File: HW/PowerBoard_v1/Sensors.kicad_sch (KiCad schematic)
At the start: 46 parts, among them U3 MCP9700AT-ETT, U4 PAMC1350DWVR, U5 PAMC1350DWVR, U6 PAMC1350DWVR, U7 PAMC1350DWVR, U8 3v3 ISO DC/DC

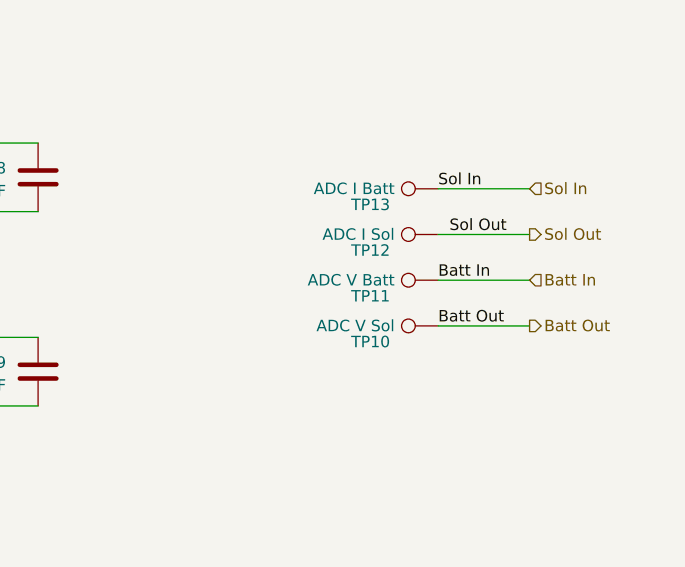
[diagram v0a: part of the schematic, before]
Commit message: pushed board
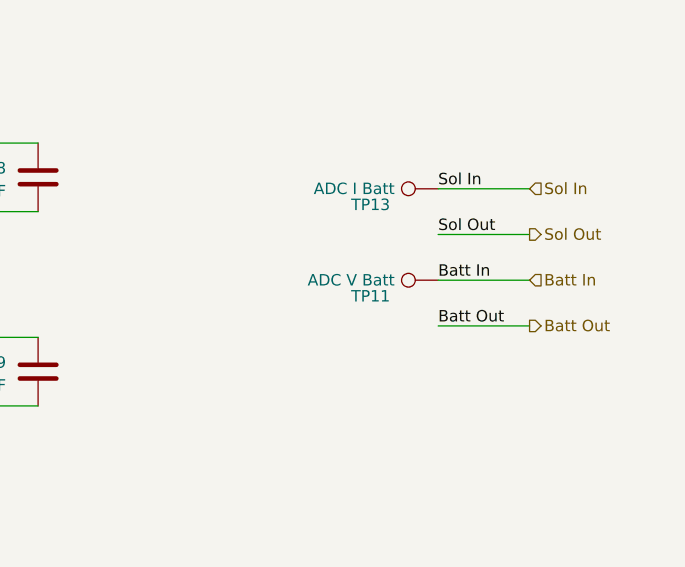
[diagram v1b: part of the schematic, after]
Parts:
- removed TP10: ADC V Sol, TestPoint:TestPoint_THTPad_1.0x1.0mm_Drill0.5mm, symbol Connector:TestPoint
- removed TP12: ADC I Sol, TestPoint:TestPoint_THTPad_1.0x1.0mm_Drill0.5mm, symbol Connector:TestPoint
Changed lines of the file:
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@@
 		)
 	)
-	(wire
-		(pts
-			(xy 245.11 129.54) (xy 255.27 129.54)
-		)
-		(stroke
-			(width 0)
-			(type default)
-		)
-	)
 	(polyline
 		(pts
@@
 	(wire
 		(pts
+			(xy 245.11 129.54) (xy 255.27 129.54)
+		)
+		(stroke
+			(width 0)
+			(type default)
+		)
+	)
+	(wire
+		(pts
 			(xy 127 87.63) (xy 116.84 87.63)
 		)
@@
 	)
 	(label "Sol Out"
-		(at 252.73 129.54 180)
+		(at 245.11 129.54 0)
 		(fields_autoplaced yes)
 		(effects
@@
 				(size 1.27 1.27)
 			)
-			(justify right bottom)
+			(justify left bottom)
 		)
 	)
@@
 	)
 	(symbol
-		(lib_id "Connector:TestPoint")
-		(at 245.11 139.7 90)
-		(unit 1)
-		(exclude_from_sim no)
-		(in_bom yes)
-		(on_board yes)
-		(dnp no)
-		(property "Reference" "TP10"
-			(at 239.776 141.478 90)
-			(effects
-				(font
-					(size 1.27 1.27)
-				)
-				(justify left)
-			)
-		)
-		(property "Value" "ADC V Sol"
-			(at 240.284 139.7 90)
-			(effects
-				(font
-					(size 1.27 1.27)
-				)
-				(justify left)
-			)
-		)
-		(property "Footprint" "TestPoint:TestPoint_THTPad_1.0x1.0mm_Drill0.5mm"
-			(at 245.11 134.62 0)
-			(effects
-				(font
-					(size 1.27 1.27)
-				)
-				(hide yes)
-			)
-		)
-		(property "Datasheet" "~"
-			(at 245.11 134.62 0)
-			(effects
-				(font
-					(size 1.27 1.27)
-				)
-				(hide yes)
-			)
-		)
-		(property "Description" "test point"
-			(at 245.11 139.7 0)
-			(effects
-				(font
-					(size 1.27 1.27)
-				)
-				(hide yes)
-			)
-		)
-		(pin "1"
-		)
-		(instances
-			(project "power_v1"
-				(path "/1e1b062d-fad0-427c-a622-c5b8a80b5268/f37b00a5-62bb-47d6-b18e-0a47b6349fc3"
-					(reference "TP10")
-					(unit 1)
-				)
-			)
-		)
-	)
-	(symbol
 		(lib_id "device:C")
 		(at 189.23 67.31 0)
@@
 					(unit 1)
 				)
-			)
-		)
-	)
-	(symbol
-		(lib_id "Connector:TestPoint")
-		(at 245.11 129.54 90)
-		(unit 1)
-		(exclude_from_sim no)
-		(in_bom yes)
-		(on_board yes)
-		(dnp no)
-		(property "Reference" "TP12"
-			(at 239.776 131.318 90)
-			(effects
-				(font
-					(size 1.27 1.27)
-				)
-				(justify left)
-			)
-		)
-		(property "Value" "ADC I Sol"
-			(at 240.284 129.54 90)
-			(effects
-				(font
-					(size 1.27 1.27)
-				)
-				(justify left)
-			)
-		)
-		(property "Footprint" "TestPoint:TestPoint_THTPad_1.0x1.0mm_Drill0.5mm"
-			(at 245.11 124.46 0)
-			(effects
-				(font
-					(size 1.27 1.27)
-				)
-				(hide yes)
-			)
-		)
-		(property "Datasheet" "~"
-			(at 245.11 124.46 0)
-			(effects
-				(font
-					(size 1.27 1.27)
-				)
-				(hide yes)
-			)
-		)
-		(property "Description" "test point"
-			(at 245.11 129.54 0)
-			(effects
-				(font
-					(size 1.27 1.27)
-				)
-				(hide yes)
-			)
-		)
-		(pin "1"
-		)
-		(instances
-			(project "power_v1"
-				(path "/1e1b062d-fad0-427c-a622-c5b8a80b5268/f37b00a5-62bb-47d6-b18e-0a47b6349fc3"
-					(reference "TP12")
-					(unit 1)
-				)
